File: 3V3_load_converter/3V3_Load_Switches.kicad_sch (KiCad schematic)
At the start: 29 parts, among them Q18 SI2302DDS-T1-GE3, Q19 SI2302DDS-T1-GE3, Q20 SI2302DDS-T1-GE3, U1 LMV321RIYLT, U2 INA199C3DCKR, U3 INA199C3DCKR, U4 INA199C1DCKR, U5 NVTFS5116PLTAG, U6 NVTFS5116PLTAG, U7 NVTFS5116PLTAG

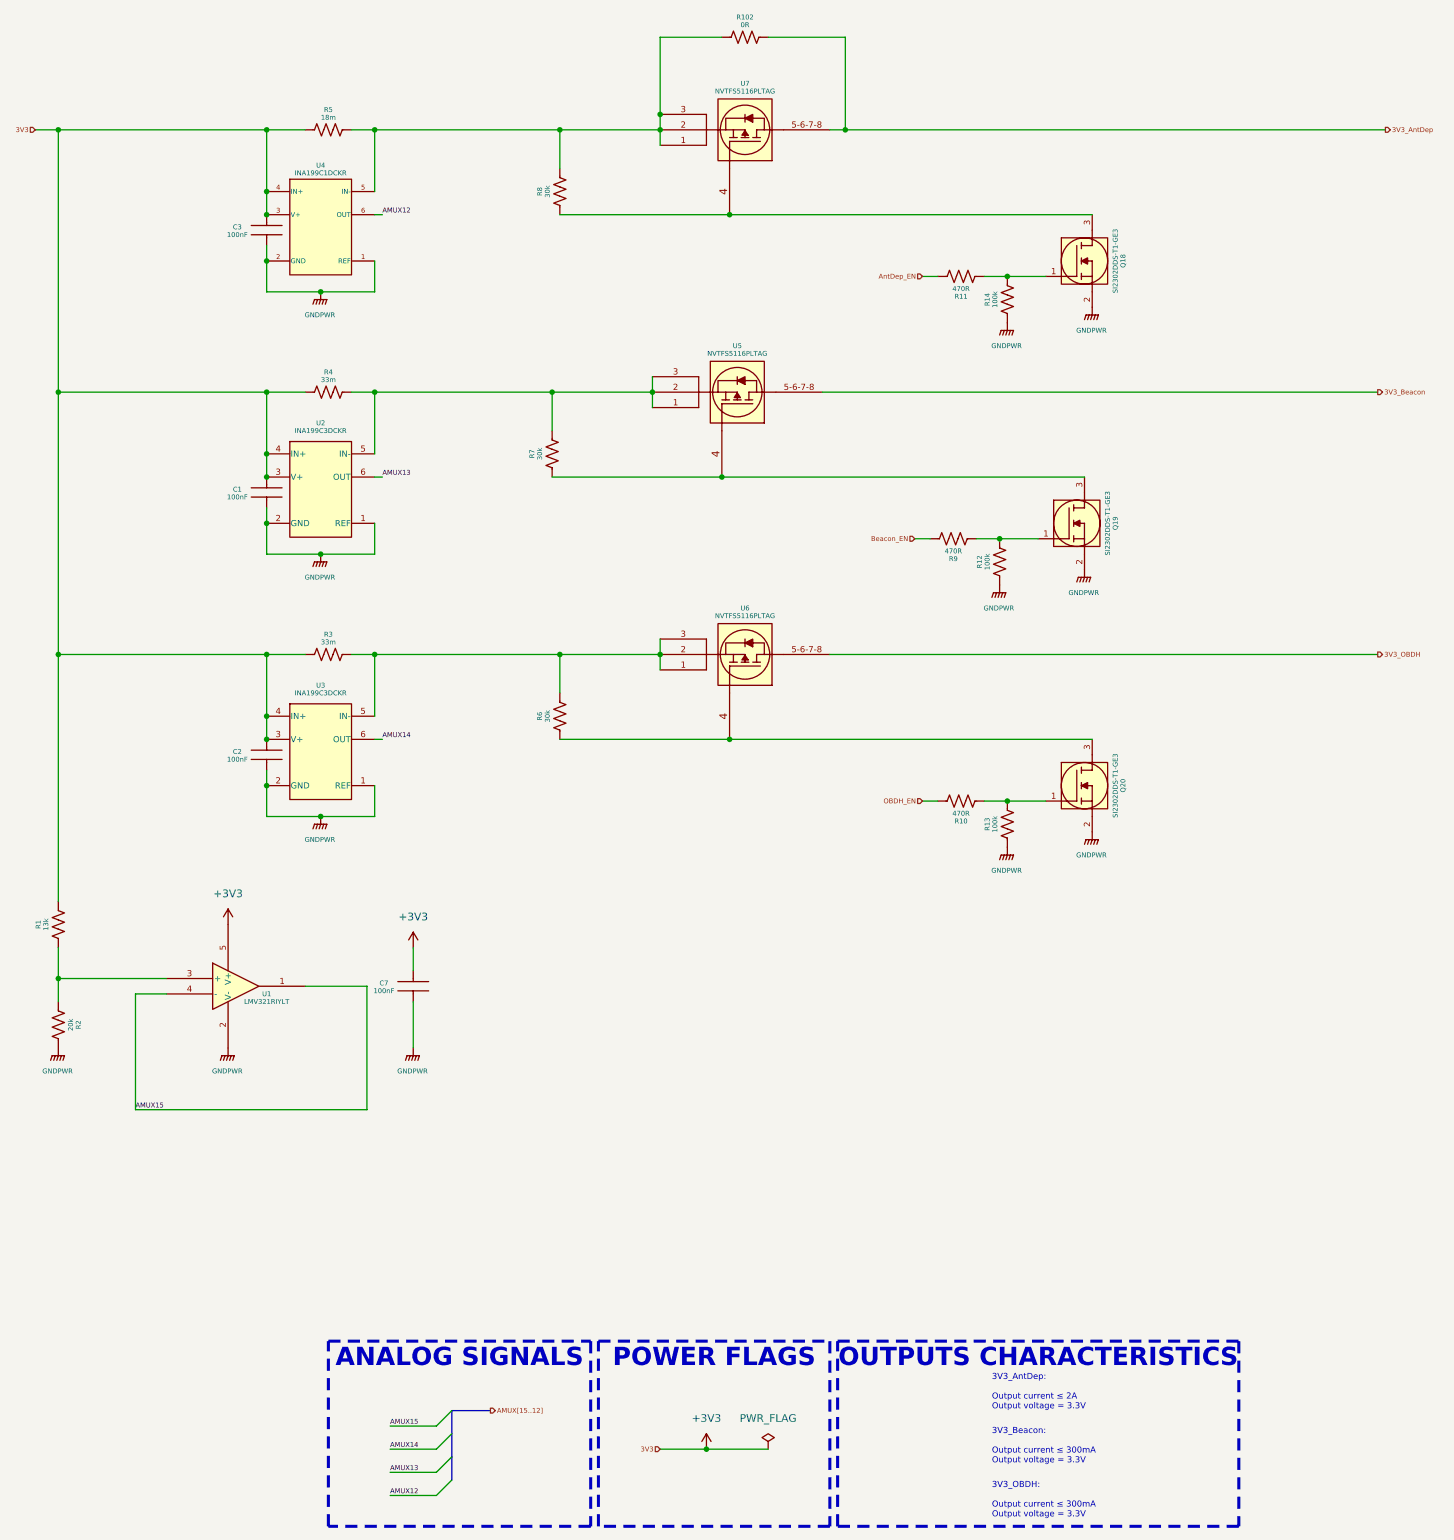
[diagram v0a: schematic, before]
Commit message: update
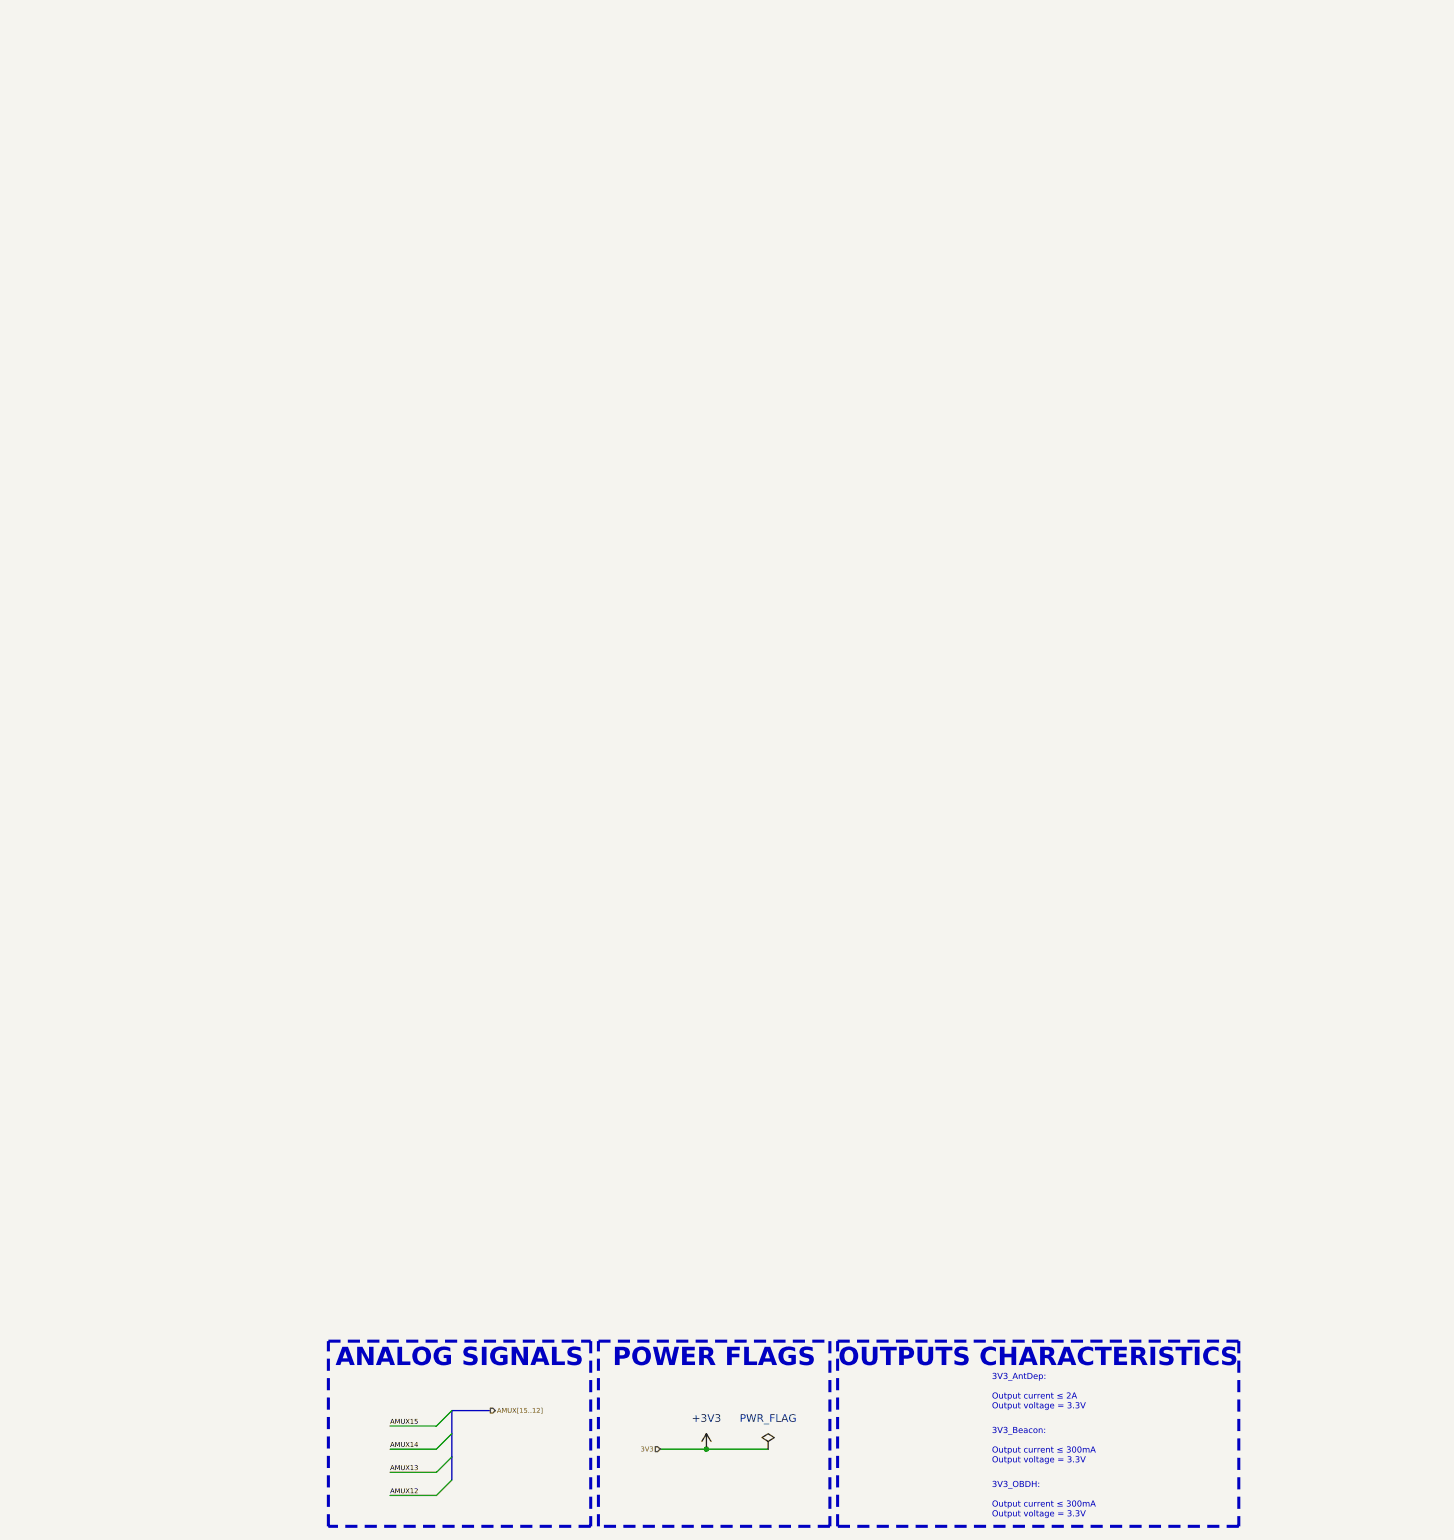
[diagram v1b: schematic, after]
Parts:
- removed C1, C2, C3, C7: 100nF, footprints:CAP0603, symbol C0603C104K5RACTU:C0603C104K5RACTU
- removed Q18, Q19, Q20: SI2302DDS-T1-GE3, footprints:SI2302DDS-T1-GE3, symbol SI2302DDS-T1-GE3:SI2302DDS-T1-GE3
- removed R1: 13k, footprints:RES0603, symbol CRCW060313K0FKEAHP:CRCW060313K0FKEAHP
- removed R10, R11, R9: 470R, footprints:RES0603, symbol CRCW0603470RFKEAHP:CRCW0603470RFKEAHP
- removed R102: 0R, footprints:RES0603, symbol CRCW06030000Z0EAHP:CRCW06030000Z0EAHP
- removed R12, R13, R14: 100k, footprints:RES0603, symbol CRCW0603100KFKEAHP:CRCW0603100KFKEAHP
- removed R2: 20k, footprints:RES0603, symbol CRCW060320K0FKEAHP:CRCW060320K0FKEAHP
- removed R3, R4: 33m, footprints:RES2010, symbol WSL2010R0330FEA:WSL2010R0330FEA
- removed R5: 18m, footprints:RES2010, symbol WSL2010R0180FEA:WSL2010R0180FEA
- removed R6, R7, R8: 30k, footprints:RES0603, symbol CRCW060330K0FKEAHP:CRCW060330K0FKEAHP
- removed U1: LMV321RIYLT, footprints:LMV321RIYLT, symbol LMV321RIYLT:LMV321RIYLT
- removed U2, U3: INA199C3DCKR, footprints:INA199C3DCKR, symbol INA199C3DCKR:INA199C3DCKR
- removed U4: INA199C1DCKR, footprints:INA199C1DCKR, symbol INA199C1DCKR:INA199C1DCKR
- removed U5, U6, U7: NVTFS5116PLTAG, footprints:NVTFS5116PLTAG, symbol NVTFS5116PLWFTAG:NVTFS5116PLTAG
